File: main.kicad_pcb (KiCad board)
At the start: 2 copper layers, 269.7 x 101.4 mm, 90 parts, among them SW1 SW_PUSH, SW10 SW_PUSH, SW11 SW_PUSH, SW12 SW_PUSH, SW13 SW_PUSH, SW14 SW_PUSH, SW15 SW_PUSH, SW16 SW_PUSH, SW17 SW_PUSH, SW18 SW_PUSH, SW19 SW_PUSH, SW2 SW_PUSH, SW20 SW_PUSH, SW21 SW_PUSH, SW22 SW_PUSH, SW23 SW_PUSH, SW24 SW_PUSH, SW25 SW_PUSH, SW26 SW_PUSH, SW27 SW_PUSH, SW28 SW_PUSH, SW29 SW_PUSH, SW3 SW_PUSH, SW30 SW_PUSH, SW31 SW_PUSH, SW32 SW_PUSH, SW33 SW_PUSH, SW34 SW_PUSH, SW35 SW_PUSH, SW36 SW_PUSH, SW37 SW_PUSH, SW38 SW_PUSH, SW39 SW_PUSH, SW4 SW_PUSH, SW40 SW_PUSH, SW41 SW_PUSH, SW42 SW_PUSH, SW43 SW_PUSH, SW44 SW_PUSH, SW5 SW_PUSH, SW6 SW_PUSH, SW7 SW_PUSH, SW8 SW_PUSH, SW9 SW_PUSH, U1 RP2040_ZERO

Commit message: :sparkles: (fix)
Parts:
- added L1: SK6812MINI-E, kamo3_footprint:YS-SK6812MINI-E, B.Cu at (26.2, 20.3)
- added L10: SK6812MINI-E, kamo3_footprint:YS-SK6812MINI-E, B.Cu at (221.4, 22.0)
- added L11: SK6812MINI-E, kamo3_footprint:YS-SK6812MINI-E, B.Cu at (244.3, 18.4)
- added L12: SK6812MINI-E, kamo3_footprint:YS-SK6812MINI-E, B.Cu at (263.4, 20.4)
- added L13: SK6812MINI-E, kamo3_footprint:YS-SK6812MINI-E, B.Cu at (26.2, 39.3)
- added L14: SK6812MINI-E, kamo3_footprint:YS-SK6812MINI-E, B.Cu at (45.3, 39.3)
- added L15: SK6812MINI-E, kamo3_footprint:YS-SK6812MINI-E, B.Cu at (66.9, 39.8)
- added L16: SK6812MINI-E, kamo3_footprint:YS-SK6812MINI-E, B.Cu at (85.4, 43.7)
- added L17: SK6812MINI-E, kamo3_footprint:YS-SK6812MINI-E, B.Cu at (104.1, 47.7)
- added L18: SK6812MINI-E, kamo3_footprint:YS-SK6812MINI-E, B.Cu at (122.8, 51.6)
- added L19: SK6812MINI-E, kamo3_footprint:YS-SK6812MINI-E, B.Cu at (175.1, 51.3)
- added L2: SK6812MINI-E, kamo3_footprint:YS-SK6812MINI-E, B.Cu at (45.3, 20.4)
- added L20: SK6812MINI-E, kamo3_footprint:YS-SK6812MINI-E, B.Cu at (193.7, 47.2)
- added L21: SK6812MINI-E, kamo3_footprint:YS-SK6812MINI-E, B.Cu at (212.3, 43.3)
- added L22: SK6812MINI-E, kamo3_footprint:YS-SK6812MINI-E, B.Cu at (230.9, 39.4)
- added L23: SK6812MINI-E, kamo3_footprint:YS-SK6812MINI-E, B.Cu at (252.8, 39.4)
- added L24: SK6812MINI-E, kamo3_footprint:YS-SK6812MINI-E, B.Cu at (271.8, 39.4)
- added L25: SK6812MINI-E, kamo3_footprint:YS-SK6812MINI-E, B.Cu at (31.0, 58.4)
- added L26: SK6812MINI-E, kamo3_footprint:YS-SK6812MINI-E, B.Cu at (50.0, 58.4)
- added L27: SK6812MINI-E, kamo3_footprint:YS-SK6812MINI-E, B.Cu at (72.2, 60.3)
- added L28: SK6812MINI-E, kamo3_footprint:YS-SK6812MINI-E, B.Cu at (90.8, 64.3)
- added L29: SK6812MINI-E, kamo3_footprint:YS-SK6812MINI-E, B.Cu at (109.5, 68.2)
- added L3: SK6812MINI-E, kamo3_footprint:YS-SK6812MINI-E, B.Cu at (66.2, 20.1)
- added L30: SK6812MINI-E, kamo3_footprint:YS-SK6812MINI-E, B.Cu at (128.1, 72.2)
- added L31: SK6812MINI-E, kamo3_footprint:YS-SK6812MINI-E, B.Cu at (167.0, 72.5)
- added L32: SK6812MINI-E, kamo3_footprint:YS-SK6812MINI-E, B.Cu at (185.6, 68.5)
- added L33: SK6812MINI-E, kamo3_footprint:YS-SK6812MINI-E, B.Cu at (204.1, 64.5)
- added L34: SK6812MINI-E, kamo3_footprint:YS-SK6812MINI-E, B.Cu at (222.7, 60.6)
- added L35: SK6812MINI-E, kamo3_footprint:YS-SK6812MINI-E, B.Cu at (244.3, 58.4)
- added L36: SK6812MINI-E, kamo3_footprint:YS-SK6812MINI-E, B.Cu at (263.3, 58.4)
- added L37: SK6812MINI-E, kamo3_footprint:YS-SK6812MINI-E, B.Cu at (74.0, 80.0)
- added L38: SK6812MINI-E, kamo3_footprint:YS-SK6812MINI-E, B.Cu at (92.5, 83.9)
- added L39: SK6812MINI-E, kamo3_footprint:YS-SK6812MINI-E, B.Cu at (111.2, 87.9)
- added L4: SK6812MINI-E, kamo3_footprint:YS-SK6812MINI-E, B.Cu at (84.8, 24.0)
- added L40: SK6812MINI-E, kamo3_footprint:YS-SK6812MINI-E, B.Cu at (129.7, 91.8)
- added L41: SK6812MINI-E, kamo3_footprint:YS-SK6812MINI-E, B.Cu at (166.3, 92.0)
- added L42: SK6812MINI-E, kamo3_footprint:YS-SK6812MINI-E, B.Cu at (185.0, 88.1)
- added L43: SK6812MINI-E, kamo3_footprint:YS-SK6812MINI-E, B.Cu at (203.4, 84.2)
- added L44: SK6812MINI-E, kamo3_footprint:YS-SK6812MINI-E, B.Cu at (222.0, 80.2)
- added L5: SK6812MINI-E, kamo3_footprint:YS-SK6812MINI-E, B.Cu at (103.4, 27.9)
- added L6: SK6812MINI-E, kamo3_footprint:YS-SK6812MINI-E, B.Cu at (122.1, 32.1)
- added L7: SK6812MINI-E, kamo3_footprint:YS-SK6812MINI-E, B.Cu at (165.6, 33.9)
- added L8: SK6812MINI-E, kamo3_footprint:YS-SK6812MINI-E, B.Cu at (184.2, 29.9)
- added L9: SK6812MINI-E, kamo3_footprint:YS-SK6812MINI-E, B.Cu at (202.8, 25.9)
- added Q1: BSS138, Package_TO_SOT_SMD:SOT-23, B.Cu at (131.7, 45.7)
- added R1: 10K, Resistor_SMD:R_1206_3216Metric_Pad1.30x1.75mm_HandSolder, B.Cu at (133.1, 39.6)
- added R2: 10K, Resistor_SMD:R_1206_3216Metric_Pad1.30x1.75mm_HandSolder, B.Cu at (130.2, 39.6)
- moved D8 9.39 mm to (191.7, 42.6)
- moved D9 9.25 mm to (210.3, 38.6)
- moved D10 9.05 mm to (229.1, 34.6)
- moved D7 8.90 mm to (173.3, 46.6)
- moved SW11 8.69 mm to (244.3, 23.4)
- moved D11 8.66 mm to (249.7, 32.5)
- moved SW10 8.63 mm to (222.4, 26.8)
- moved D12 8.60 mm to (268.7, 34.3)
- moved SW9 8.57 mm to (203.8, 30.8)
- moved SW8 8.54 mm to (185.2, 34.7)
- moved SW12 8.53 mm to (263.3, 25.3)
- moved SW7 8.48 mm to (166.7, 38.8)
- moved SW40 5.84 mm to (128.7, 96.7)
- moved SW39 5.79 mm to (110.1, 92.7)
- moved SW37 5.77 mm to (72.9, 84.8)
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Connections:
- U1 pad 10: /col6 -> /col9
- U1 pad 11: unconnected-(U1-GP10-Pad11) -> /col2
- U1 pad 12: unconnected-(U1-GP11-Pad12) -> /col3
- U1 pad 13: unconnected-(U1-GP12-Pad13) -> /col4
- U1 pad 14: unconnected-(U1-GP13-Pad14) -> /col5
- U1 pad 15: /col5 -> unconnected-(U1-GP14-Pad15)
- U1 pad 16: /col4 -> unconnected-(U1-GP15-Pad16)
- U1 pad 17: /col3 -> unconnected-(U1-GP26-Pad17)
- U1 pad 18: /col2 -> /col1
- U1 pad 19: /col1 -> /col0
- U1 pad 20: /col0 -> /led_v3.3
- U1 pad 7: /col9 -> /col6
- U1 pad 8: /col8 -> /col7
- U1 pad 9: /col7 -> /col8
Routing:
- net VDC: track 0.00 -> 1156.2 mm
- net Net-(L24-DOUT): track 0.00 -> 285.6 mm, vias 0 -> 2
- net Net-(L12-DOUT): track 0.00 -> 280.4 mm, vias 0 -> 2
- net Net-(L36-DOUT): track 0.00 -> 241.7 mm, vias 0 -> 2
- net /led_v5: track 0.00 -> 138.1 mm, vias 0 -> 2
- net /row3: track 530.1 -> 427.4 mm, vias 0 -> 2
- net /col2: track 172.1 -> 237.3 mm, vias 4 -> 5
- net /col7: track 121.8 -> 180.0 mm, vias 4 -> 5
- net /col9: track 157.6 -> 215.3 mm, vias 4 -> 5
- net /col3: track 153.3 -> 209.4 mm, vias 4 -> 5
- net /col4: track 135.9 -> 191.3 mm, vias 4 -> 5
- net /col8: track 138.2 -> 191.6 mm, vias 4 -> 5
- net /col5: track 117.4 -> 167.2 mm, vias 4 -> 5
- net Net-(L18-DOUT): track 0.00 -> 48.8 mm
- net Net-(L6-DOUT): track 0.00 -> 47.2 mm, vias 0 -> 2
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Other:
- board size 269.7 x 101.4 mm -> 269.7 x 101.9 mm

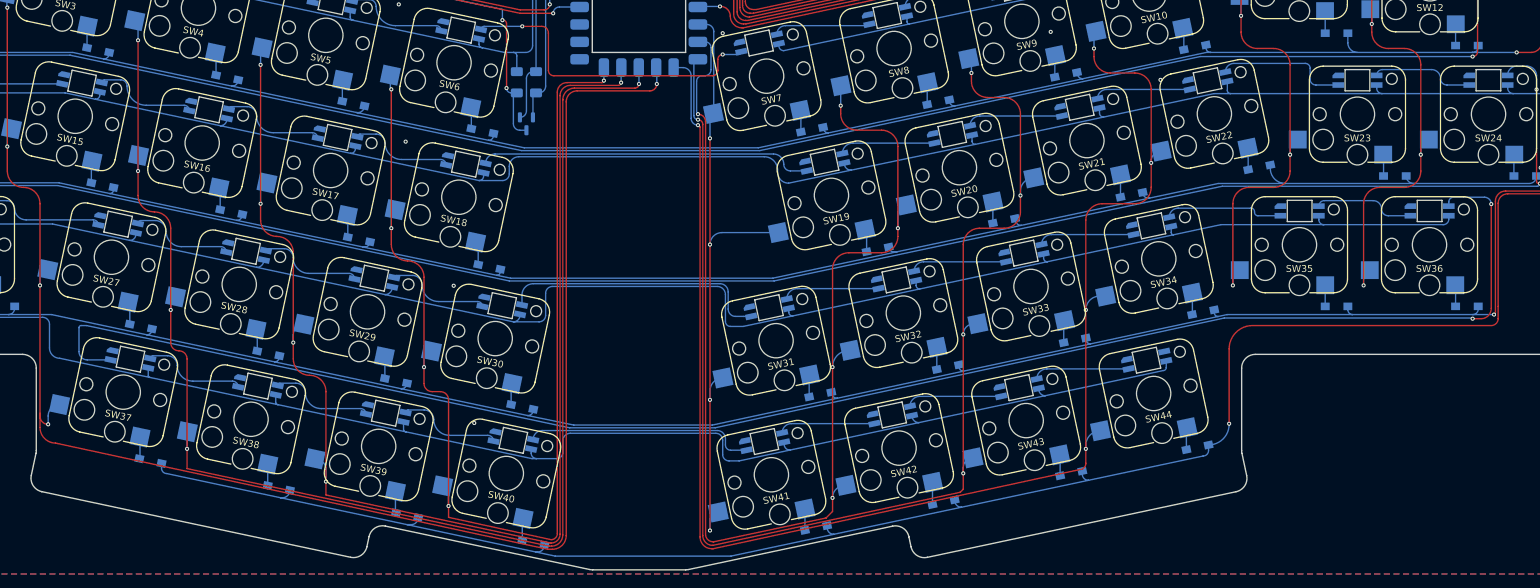
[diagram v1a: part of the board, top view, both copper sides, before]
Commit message: update
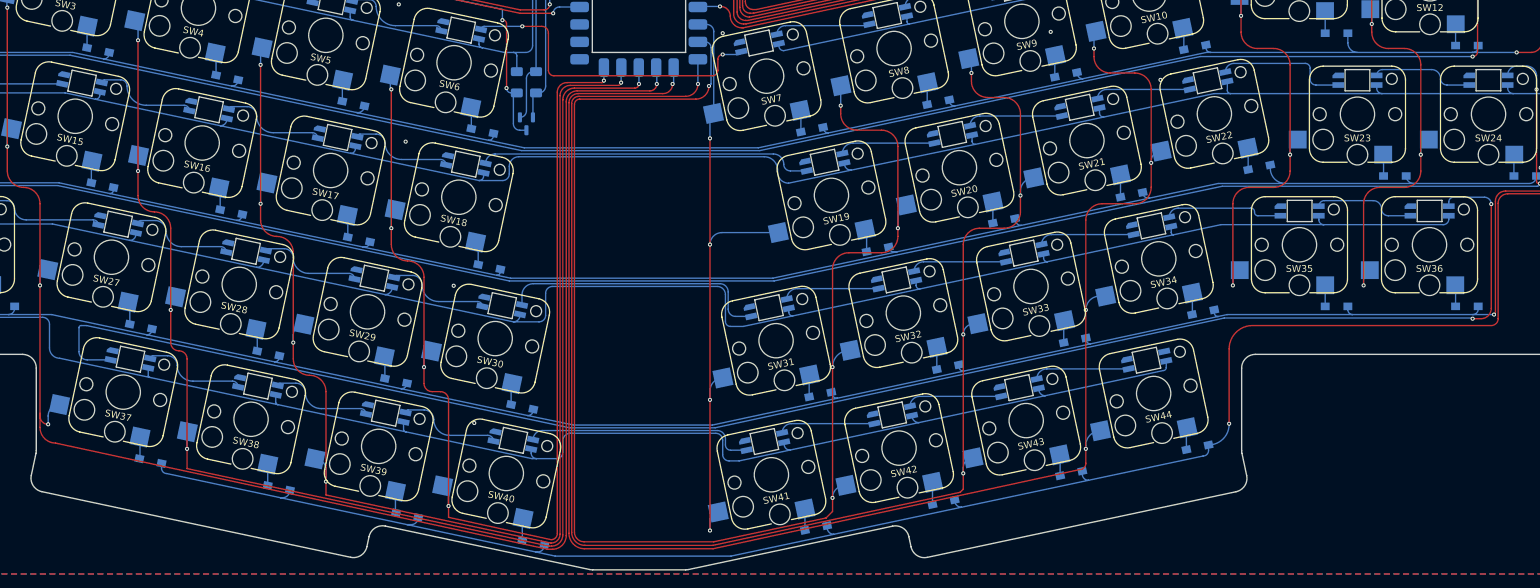
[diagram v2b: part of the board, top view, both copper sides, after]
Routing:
- net /col8: track 191.6 -> 227.5 mm
- net /col7: track 180.0 -> 215.5 mm
- net /col9: track 215.3 -> 245.4 mm
